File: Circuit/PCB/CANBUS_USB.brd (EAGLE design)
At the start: 63.5 x 69.5 mm, 22 parts

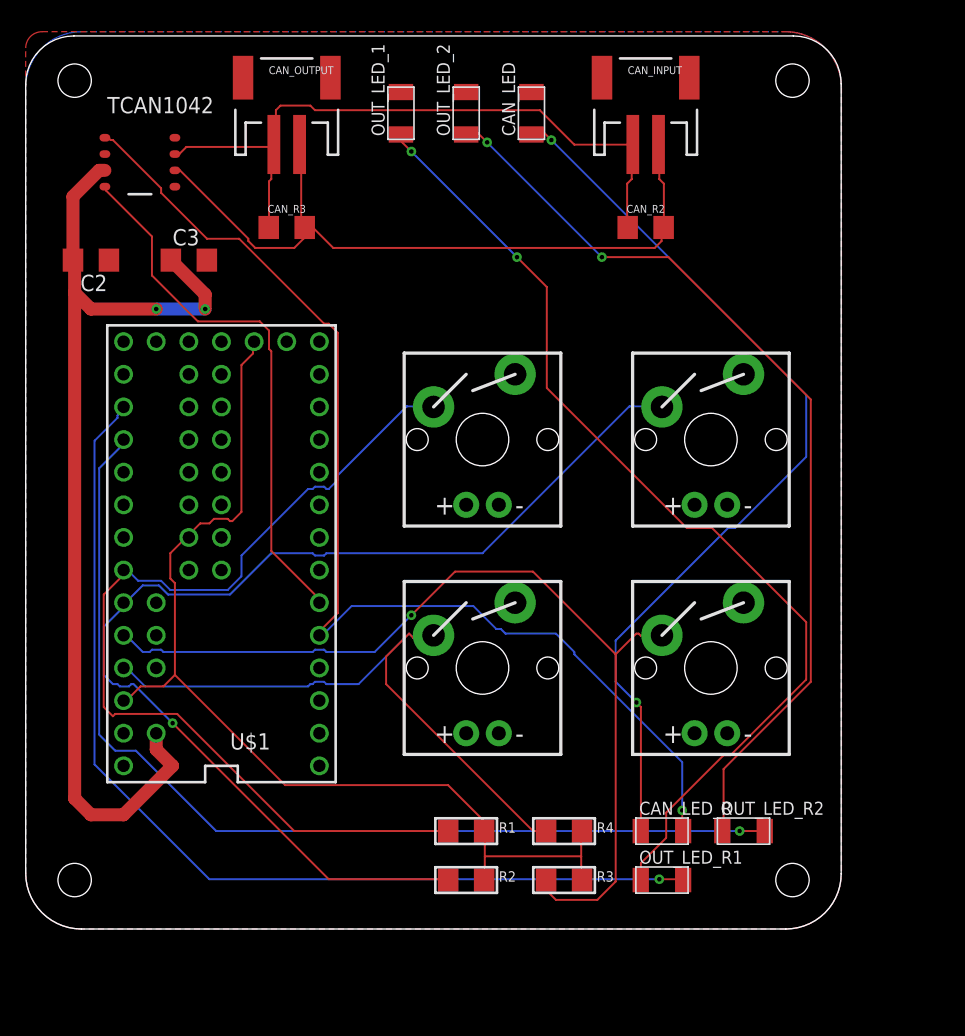
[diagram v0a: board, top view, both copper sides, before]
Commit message: PCB
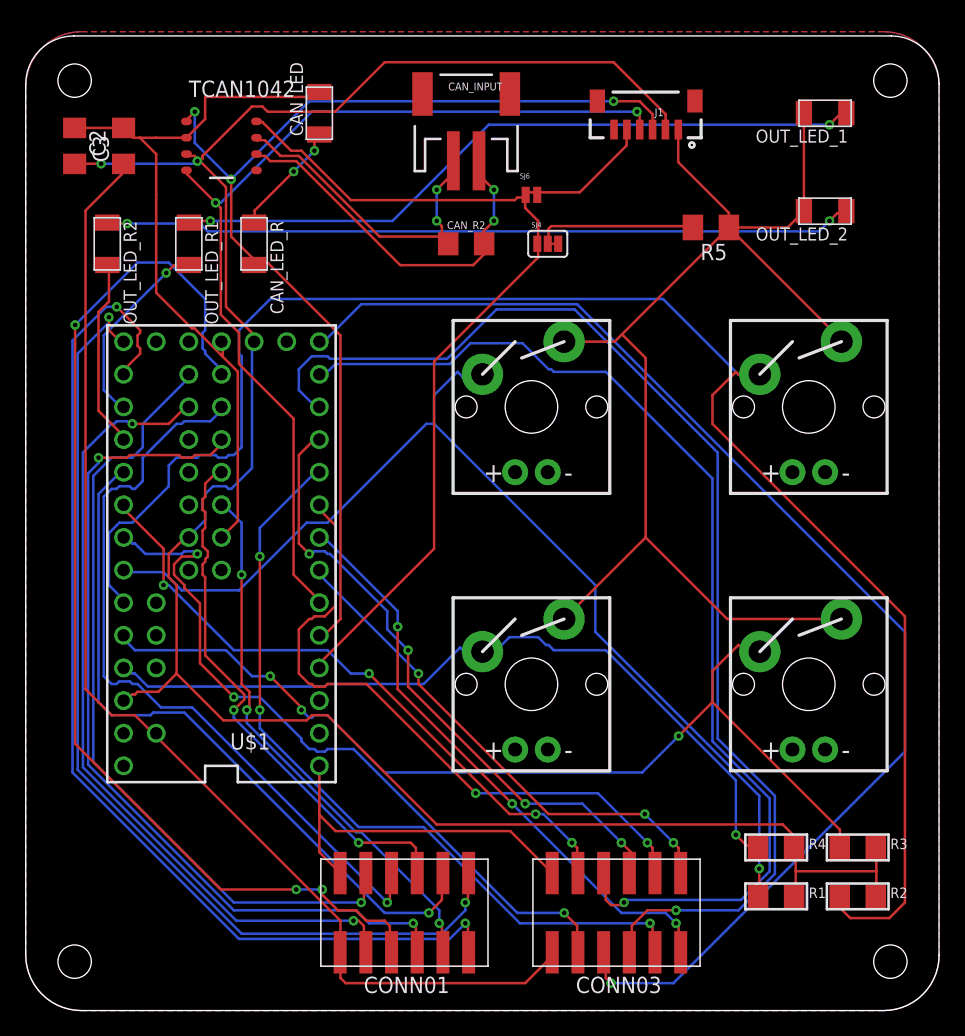
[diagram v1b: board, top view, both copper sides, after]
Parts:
- removed CAN_OUTPUT: (no value), SparkFun-Connectors:JST-2-SMD
- removed CAN_R3: 120ohm, SparkFun-Resistors:1206
- added CONN01, CONN03: TMMH-105-12, TMMH-105-XX-XX-DV:TMMH-105-12
- added J1: (no value), SparkFun-Connectors:1X06-1MM
- added R5: 10k, resistor:M1206
- added SJ4: (no value), SparkFun-Passives:PAD-JUMPER-3-2OF3_NC_BY_TRACE_YES_SILK_FULL_BOX
- added SJ6: A-VCC1, SparkFun-Passives:PAD-JUMPER-2-NO_NO_SILK
- moved OUT_LED_R2 67.4 mm to (6.35, 57.1), turned to 270 degrees
- moved OUT_LED_R1 61.7 mm to (12.7, 57.1), turned to 270 degrees
- moved CAN_LED_R 55.7 mm to (17.8, 57.1), turned to 270 degrees
- moved OUT_LED_1 33.0 mm to (62.2, 67.3), turned to 180 degrees
- moved R2 30.5 mm to (64.8, 6.35)
- moved OUT_LED_2 29.0 mm to (62.2, 59.7), turned to 180 degrees
- moved R1 24.7 mm to (58.4, 6.35)
- moved R3 23.0 mm to (64.8, 10.2)
- moved R4 16.6 mm to (58.4, 10.2)
- moved CAN_LED 16.5 mm to (22.9, 67.3)
- moved CAN_INPUT 14.0 mm to (34.3, 67.3)
- moved CAN_R2 14.0 mm to (34.3, 57.1)
- moved C3 10.2 mm to (7.62, 64.8), turned to 90 degrees
- moved C2 8.98 mm to (3.81, 64.8), turned to 270 degrees
- moved S2 8.03 mm to (61.0, 44.5)
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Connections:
- new net GPIO_01: CONN03.1, U$1.5
- new net GPIO_02: CONN03.2, U$1.6
- new net GPIO_03: CONN03.3, U$1.7
- new net GPIO_04: CONN03.4, U$1.8
- new net GPIO_05: CONN03.5, U$1.9
- new net GPIO_06: CONN03.6, U$1.10
- new net GPIO_07: CONN03.7, U$1.11
- new net GPIO_08: CONN03.8, U$1.12
- new net GPIO_09: CONN03.9, U$1.18/A4
- new net GPIO_10: CONN03.10, U$1.19/A5
- new net GPIO_11: CONN01.1, U$1.13
- new net GPIO_12: CONN01.2, U$1.14/A0
- new net GPIO_13: CONN01.3, U$1.17/A3
- new net GPIO_14: CONN01.4, U$1.24
- new net GPIO_15: CONN01.5, U$1.25
- new net GPIO_16: CONN01.6, U$1.26
- new net GPIO_17: CONN01.7, U$1.27
- new net GPIO_18: CONN01.8, U$1.28
- new net GPIO_19: CONN01.9, U$1.29
- new net GPIO_20: CONN01.10, U$1.30
- new net N$17: R5.2, SJ4.2
- new net N$20: U$1.31
- new net N$22: J1.6
- net 3.3V: now also C2.2, J1.2, TCAN1042.3
- net CAN_H: no longer CAN_OUTPUT.1, CAN_R3.1
- net CAN_L: no longer CAN_OUTPUT.2, CAN_R3.2
- net CAN_RX: now also J1.4
- net CAN_STB: now also J1.5, SJ4.1, SJ4.3, SJ6.1, SJ6.2, U$1.2
- net CAN_TX: now also J1.3
- net GND_MCU: now also CONN01.12, CONN03.12, J1.1, R5.1
- net VCC_MCU: now also CONN01.11, CONN03.11; no longer C2.2, TCAN1042.3
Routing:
- net GND_MCU: track 0.00 -> 182.7 mm
- net GPIO_08: track 0.00 -> 99.7 mm, vias 0 -> 1
- net 3.3V: track 80.2 -> 173.8 mm, vias 0 -> 2
- net GPIO_06: track 0.00 -> 92.7 mm, vias 0 -> 1
- net GPIO_18: track 0.00 -> 85.2 mm, vias 0 -> 3
- net GPIO_07: track 0.00 -> 84.7 mm, vias 0 -> 1
- net GPIO_12: track 0.00 -> 83.7 mm, vias 0 -> 2
- net CAN_STB: track 0.00 -> 79.3 mm
- net GPIO_11: track 0.00 -> 78.0 mm, vias 0 -> 2
- net GPIO_16: track 0.00 -> 67.6 mm, vias 0 -> 2
- net LED_16: track 78.7 -> 14.9 mm, vias 1 -> 0
- net GPIO_20: track 0.00 -> 63.5 mm, vias 0 -> 2
- net LED_15: track 78.4 -> 15.3 mm
- net GPIO_19: track 0.00 -> 62.2 mm, vias 0 -> 1
- net N$193: track 71.1 -> 9.01 mm
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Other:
- board size 63.5 x 69.5 mm -> 71.1 x 75.9 mm

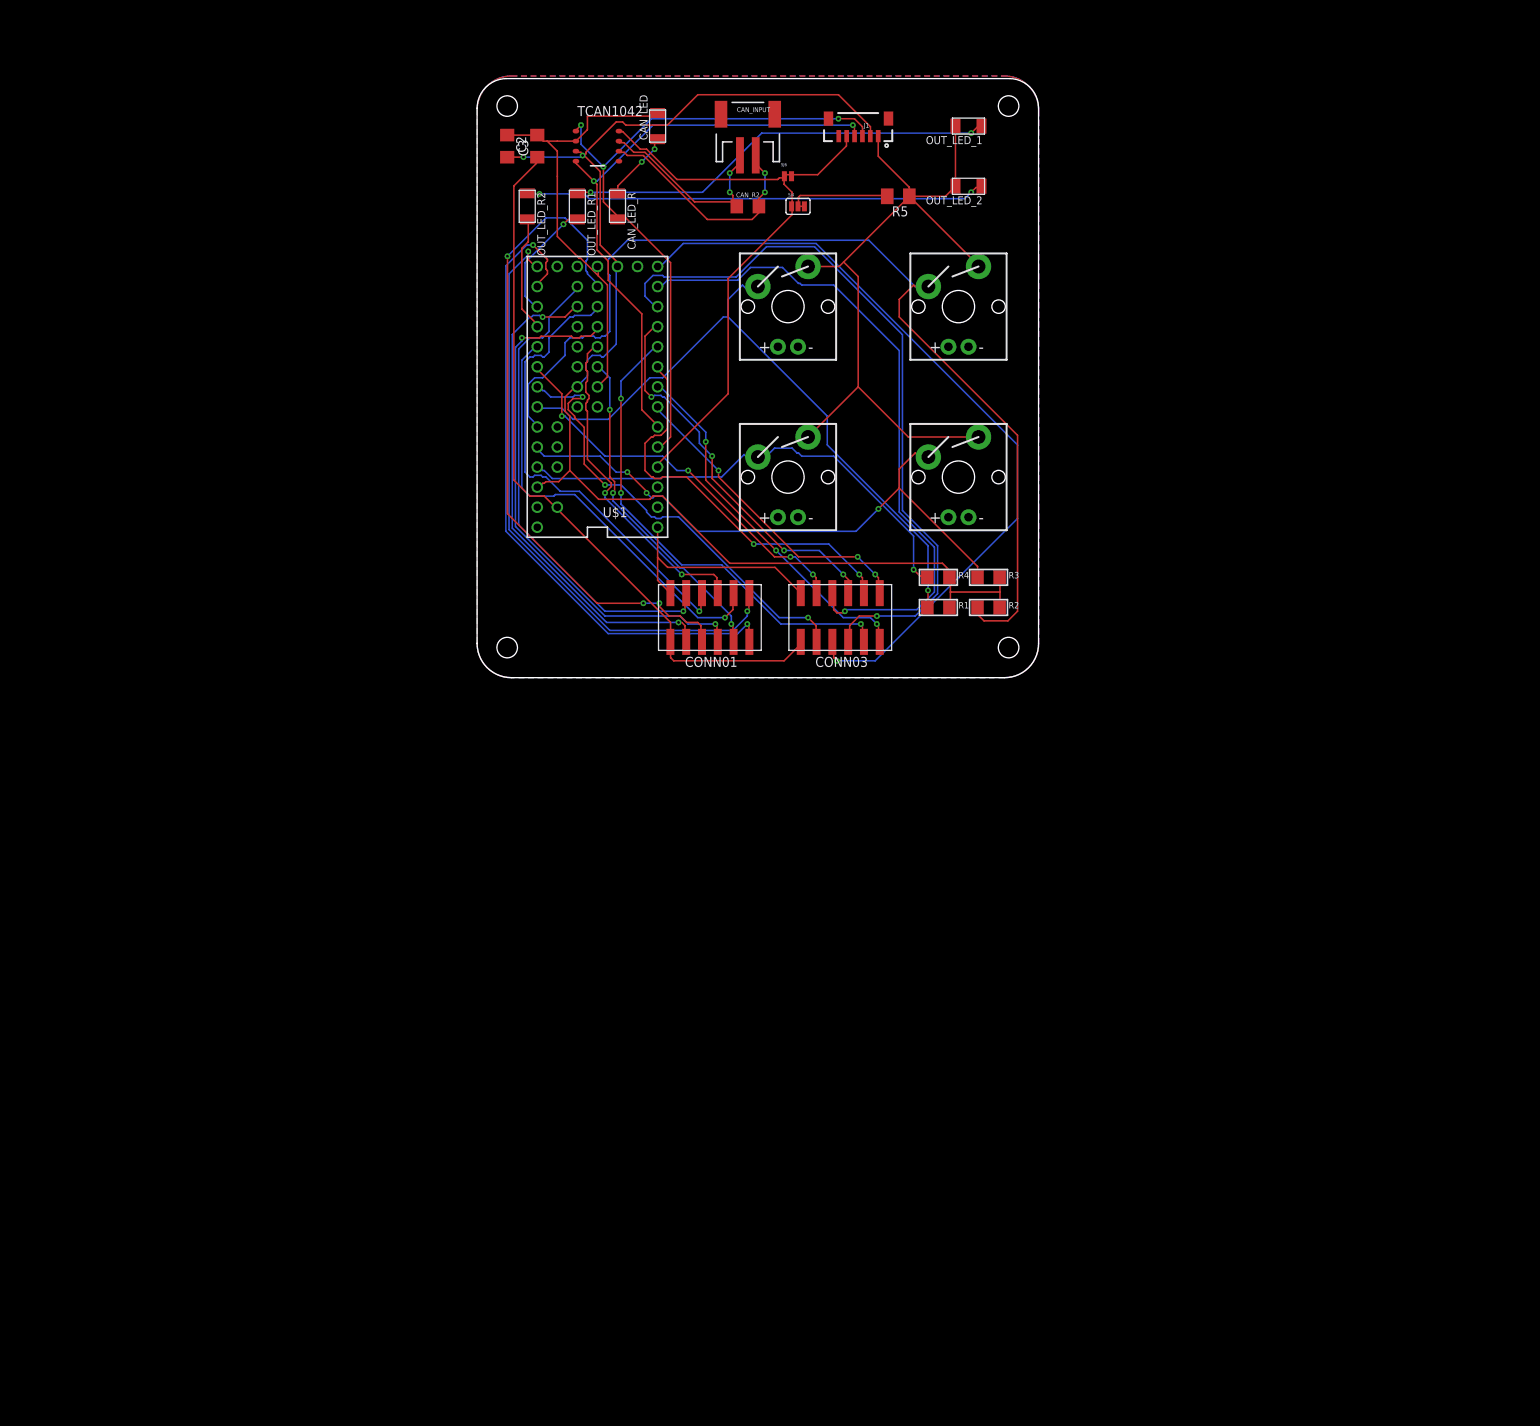
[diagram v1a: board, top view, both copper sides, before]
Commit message: components
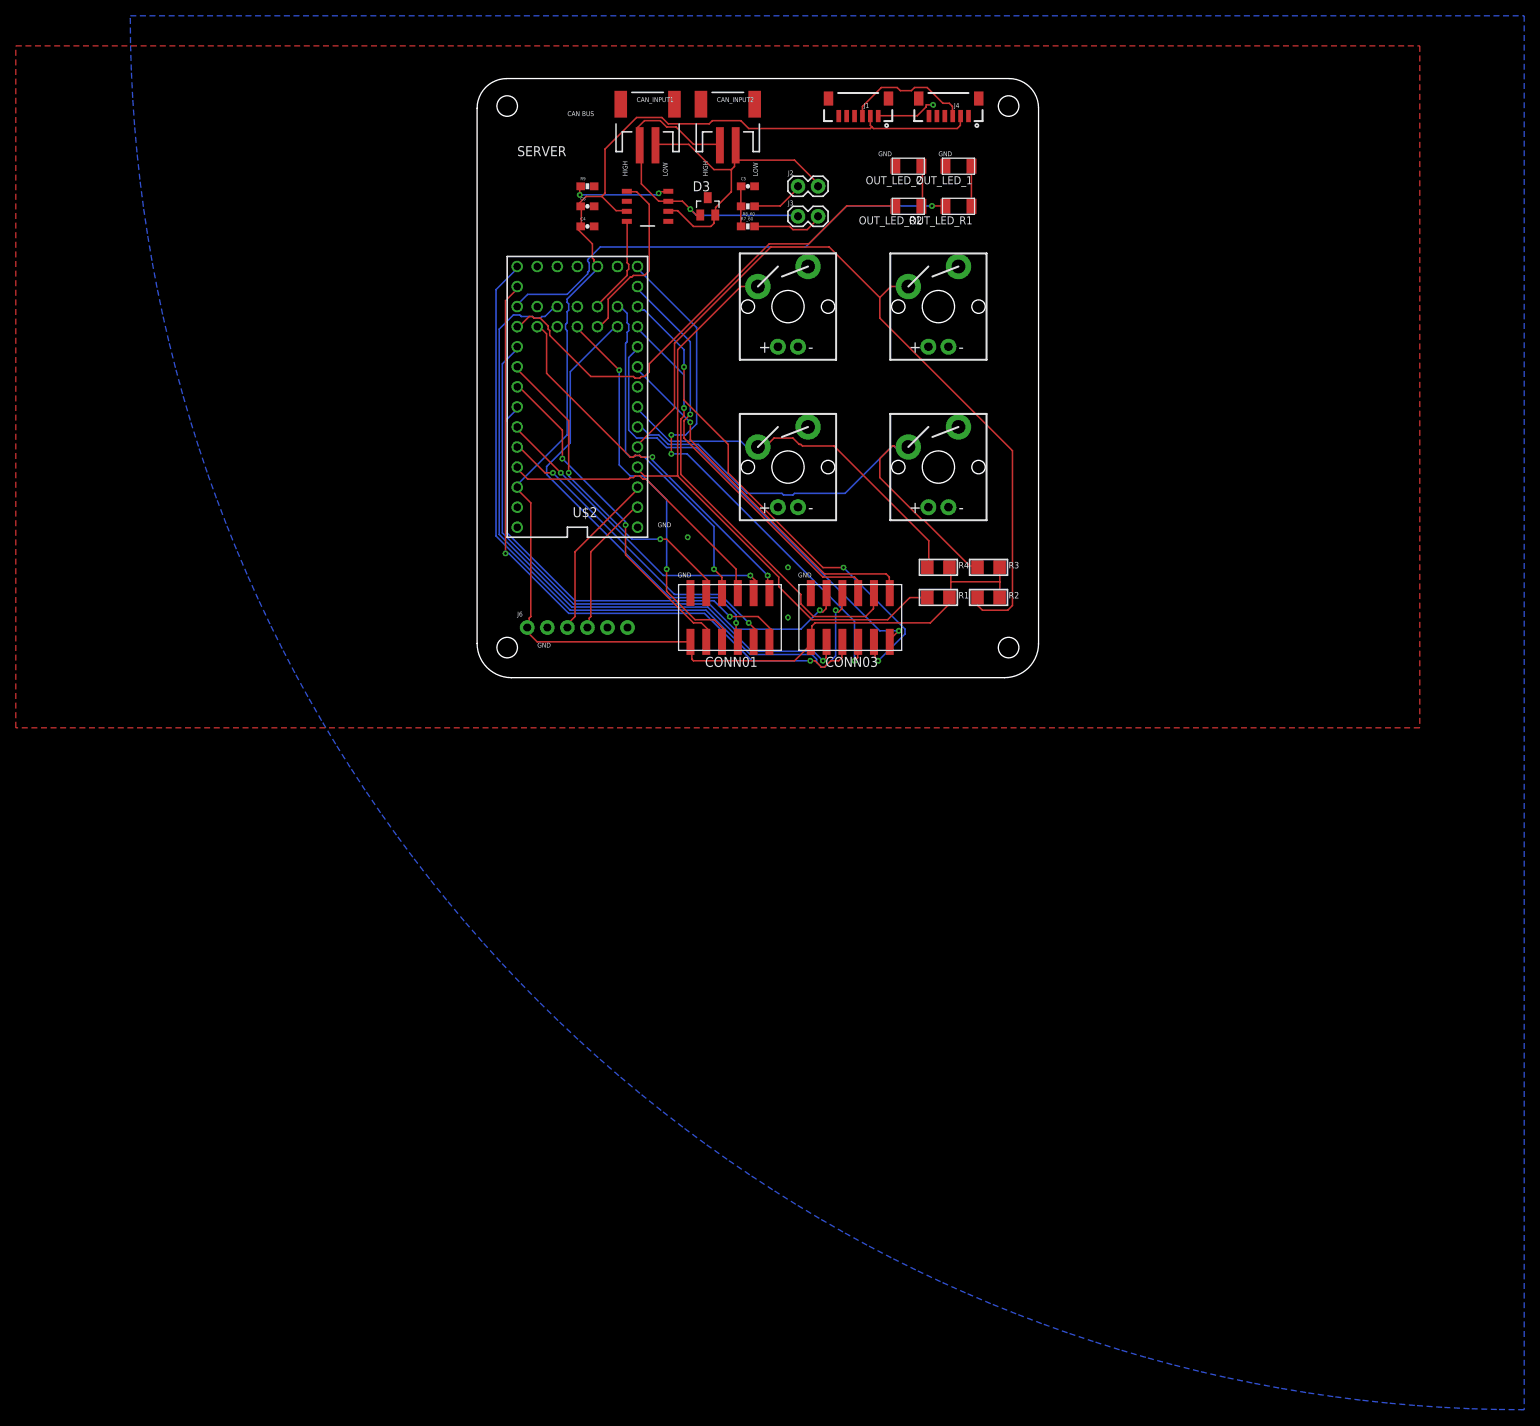
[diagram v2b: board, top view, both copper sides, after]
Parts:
- removed C2, C3: 0.1uF, adafruit:C1206
- removed CAN_INPUT: (no value), SparkFun-Connectors:JST-2-SMD
- removed CAN_LED: LEDFAB1206, fab:LED1206FAB
- removed CAN_LED_R: 500, fab:R1206FAB
- removed CAN_R2: 120ohm, SparkFun-Resistors:1206
- removed R5: 10k, resistor:M1206
- removed SJ4: (no value), SparkFun-Passives:PAD-JUMPER-3-2OF3_NC_BY_TRACE_YES_SILK_FULL_BOX
- removed SJ6: A-VCC1, SparkFun-Passives:PAD-JUMPER-2-NO_NO_SILK
- removed TCAN1042: Value, TCAN1042DRQ1:D0008A_N
- removed U$1: TEENSY_3.1-3.2_ALL_PINS&PADS, Teensy_3_and_LC_Series_Boards_v1.4:TEENSY_3.0-3.2_ALL_PINS_&_PADS
- added C4: 2.2uf, SparkFun-Capacitors:0603-CAP
- added C5: 4.7uf, SparkFun-Capacitors:0603-CAP
- added C6: 0.1uf, SparkFun-Capacitors:0603-CAP
- added CAN_INPUT1, CAN_INPUT2: (no value), SparkFun-Connectors:JST-2-SMD
- added D3: PESD1CAN, diode:SOT23
- added J2, J3: (no value), SparkFun-Connectors:1X02
- added J4: (no value), SparkFun-Connectors:1X06-1MM
- added J6: (no value), SparkFun-Connectors:1X06_NO_SILK
- added R7_60, R8_60: 60, SparkFun-Resistors:0603-RES
- added R9: 10K, SparkFun-Resistors:0603-RES
- added U$2: TEENSY_4.0_WITH_SMD_HEADER_PINS, Teensy4:TEENSY_4.0_WITH_SMD_HEADER_PINS
- added U$3: SN65HVD232Q, TCAN1042DRQ1:SN65HVD232Q
- moved OUT_LED_R1 48.3 mm to (61.0, 57.1), turned to 180 degrees
- moved OUT_LED_R2 48.3 mm to (54.6, 57.1), turned to 180 degrees
- moved OUT_LED_2 8.03 mm to (54.6, 62.2)
- moved OUT_LED_1 5.24 mm to (61.0, 62.2)
- moved S3 2.84 mm to (58.4, 24.1)
- moved CONN01 2.54 mm to (31.8, 5.08)
- moved S2 2.54 mm to (58.4, 44.5)
- moved J1 2.54 mm to (48.3, 69.8)
- moved CONN03 1.27 mm to (47.0, 5.08)
- moved R1 1.27 mm to (58.4, 7.62)
- moved R2 1.27 mm to (64.8, 7.62)
- moved R3 1.27 mm to (64.8, 11.4)
- moved R4 1.27 mm to (58.4, 11.4)
- moved S4 1.27 mm to (39.4, 24.1)
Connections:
- net N$22 renamed SWITCH_01
- removed net AGND: U$1.AGND
- removed net AREF: U$1.AREF
- removed net CAN_H: CAN_INPUT.1, CAN_R2.1, TCAN1042.7
- removed net CAN_L: CAN_INPUT.2, CAN_R2.2, TCAN1042.6
- removed net N$17: R5.2, SJ4.2
- removed net N$193: CAN_LED.1, CAN_LED_R.1
- removed net N$20: U$1.31
- removed net VCC_MCU: C3.1, CONN01.11, CONN03.11, U$1.VUSB
- new net CAN_H1: CAN_INPUT1.1, CAN_INPUT2.1, D3.1, J3.1, U$3.CANH
- new net CAN_H2: J6.5
- new net CAN_L1: CAN_INPUT1.2, CAN_INPUT2.2, D3.2, J2.2, U$3.CANL
- new net CAN_L2: J6.6
- new net CAN_RX2: J6.4, U$2.0
- new net CAN_RX3: U$2.30, U$3.R
- new net CAN_TX2: J6.3, U$2.1
- new net CAN_TX3: U$2.31, U$3.D
- new net GPIO_SCL: CONN01.10, U$2.19/A5
- new net GPIO_SDA: CONN01.9, U$2.18/A4
- new net LED_IN: J1.4
- new net N$10: U$2.24
- new net N$13: C5.1, R7_60.1, R8_60.2
- new net N$14: J2.1, R8_60.1
- new net N$28: U$2.6
- new net N$5: U$3.VREF
- new net N$6: R9.1, U$3.RS
- new net N$7: J3.2, R7_60.2
- new net SWITCH_02: J1.5
- net 3.3V: now also C4.1, C6.1, CONN01.11, CONN03.11, J4.2, J6.1, U$2.3.3V, U$2.3.3V1, U$3.VCC; no longer C2.2, TCAN1042.3, U$1.3.3V, U$1.3.3V1, U$1.3.3V2
- net CAN_RX: now also J4.4; no longer J1.4, TCAN1042.4, U$1.4
- net CAN_STB: now also J4.5; no longer J1.5, SJ4.1, SJ4.3, SJ6.1, SJ6.2, TCAN1042.8, U$1.2
- net CAN_TX: now also J4.3; no longer CAN_LED_R.2, TCAN1042.1, U$1.3
- net GND_MCU: now also C4.2, C5.2, C6.2, D3.3, J4.1, J6.2, R9.2, U$2.GND, U$2.GND1, U$2.GND2, U$3.GND; no longer C2.1, C3.2, CAN_LED.2, R5.1, TCAN1042.2, U$1.GND, U$1.GND1, U$1.GND2
- net GPIO_01: now also U$2.7; no longer U$1.5
- net GPIO_02: now also U$2.8; no longer U$1.6
- net GPIO_03: now also U$2.9; no longer U$1.7
- net GPIO_04: now also U$2.10; no longer U$1.8
- net GPIO_05: now also U$2.11; no longer U$1.9
- net GPIO_06: now also U$2.12; no longer U$1.10
- net GPIO_07: now also U$2.13; no longer U$1.11
- net GPIO_08: now also U$2.14/A0; no longer U$1.12
- net GPIO_09: now also U$2.17/A3; no longer U$1.18/A4
- net GPIO_10: now also U$2.26; no longer U$1.19/A5
- net GPIO_11: now also U$2.25; no longer U$1.13
- net GPIO_12: now also U$2.20/A6; no longer U$1.14/A0
- net GPIO_13: now also U$2.21/A7; no longer U$1.17/A3
- net GPIO_14: now also U$2.22/A8; no longer U$1.24
- net GPIO_15: now also U$2.23/A9; no longer U$1.25
- net GPIO_16: now also U$2.33; no longer U$1.26
- net GPIO_17: now also U$2.32; no longer U$1.27
- net GPIO_18: now also U$2.29; no longer U$1.28
- net GPIO_19: now also U$2.28; no longer CONN01.9, U$1.29
- net GPIO_20: now also U$2.27; no longer CONN01.10, U$1.30
- net KEY_01: now also U$2.2; no longer U$1.20/A6
- net KEY_02: now also U$2.3; no longer U$1.21/A7
- net KEY_03: now also U$2.4; no longer U$1.22/A8
- net KEY_04: now also U$2.5; no longer U$1.23/A9
- net LED_15: now also U$2.15/A1; no longer U$1.15/A1
- net LED_16: now also U$2.16/A2; no longer U$1.16/A2
- net N$2: now also J4.6; no longer U$1.VIN
- net N$3: now also U$2.VIN; no longer TCAN1042.5
- net VBAT: now also U$2.VBAT; no longer U$1.VBAT
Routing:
- net GND_MCU: track 182.7 -> 7.68 mm, vias 0 -> 4
- net VCC_MCU: track 92.1 -> 0.00 mm
- net CAN_STB: track 79.3 -> 0.00 mm
- net CAN_RX: track 75.2 -> 0.00 mm, vias 2 -> 0
- net CAN_TX: track 85.3 -> 16.2 mm, vias 3 -> 0
- net GPIO_20: track 63.5 -> 0.00 mm, vias 2 -> 0
- net GPIO_19: track 62.2 -> 0.00 mm, vias 1 -> 0
- net N$1: track 58.5 -> 5.29 mm, vias 2 -> 0
- net N$4: track 54.7 -> 5.08 mm, vias 2 -> 0
- net LED_16: track 14.9 -> 61.9 mm
- net LED_15: track 15.3 -> 60.9 mm
- net GPIO_SCL: track 0.00 -> 43.2 mm, vias 0 -> 2
- net CAN_L1: track 0.00 -> 43.0 mm
- net CAN_H1: track 0.00 -> 42.6 mm, vias 0 -> 1
- net GPIO_SDA: track 0.00 -> 41.4 mm, vias 0 -> 2
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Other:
- board text added: "CAN BUS"
- board text added: "GND"
- board text added: "HIGH"
- board text added: "LOW"
- board text added: "SERVER"
